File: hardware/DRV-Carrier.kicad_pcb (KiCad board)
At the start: 4 copper layers, 95 x 79.9 mm, 22 parts, among them J1 Conn_01x02, J2 Conn_02x25_Counter_Clockwise

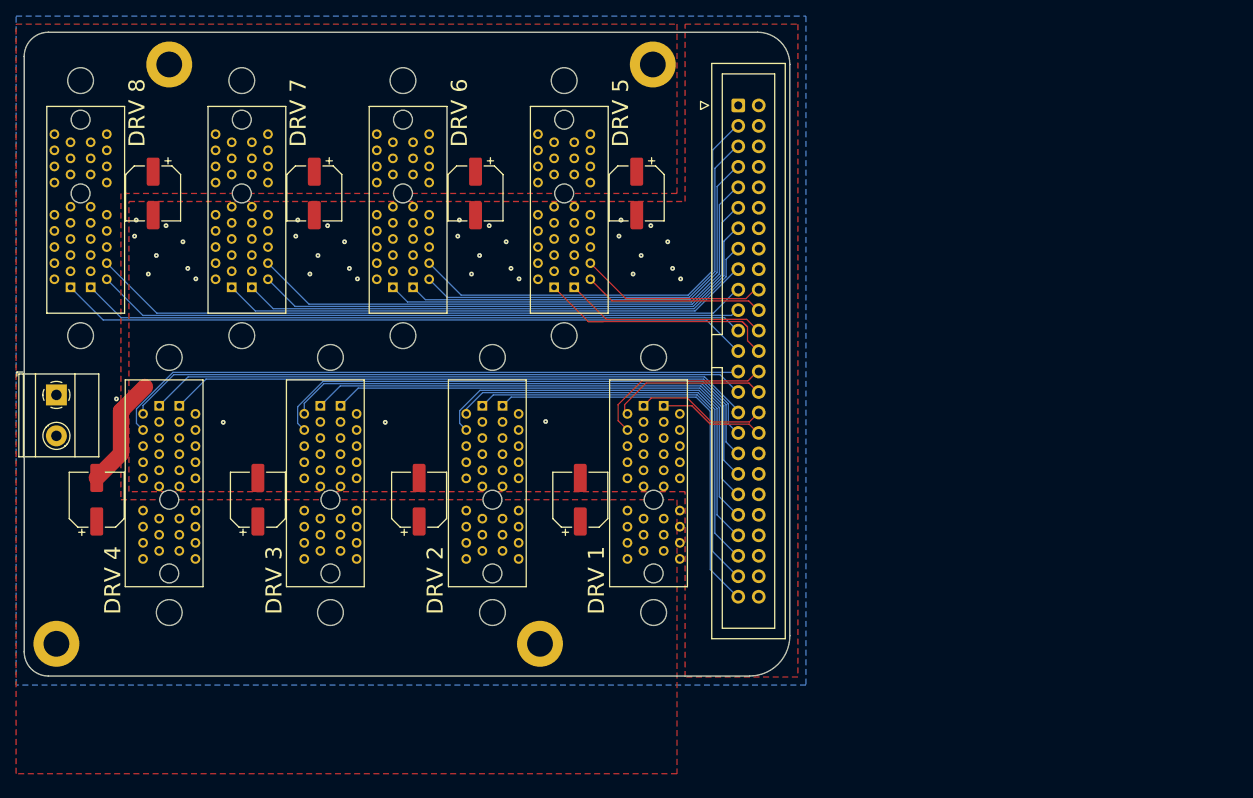
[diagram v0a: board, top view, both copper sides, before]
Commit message: V3 added
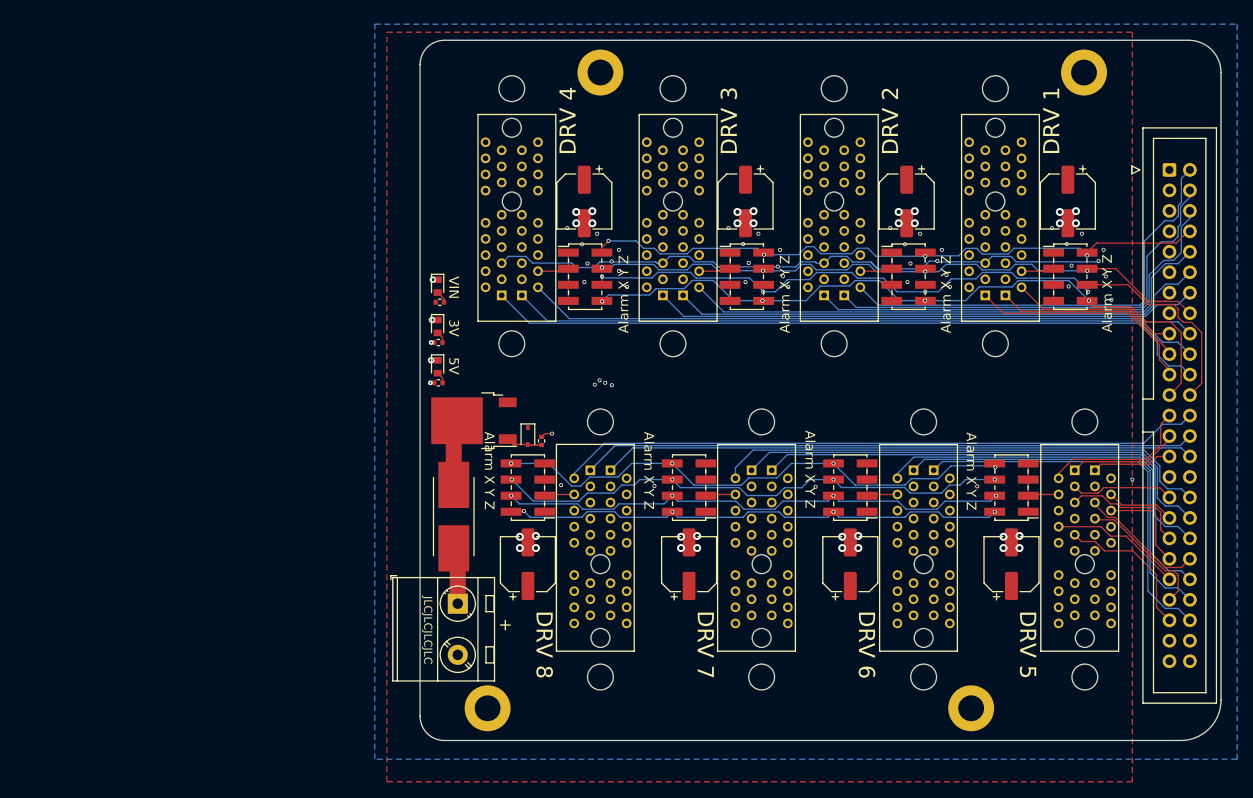
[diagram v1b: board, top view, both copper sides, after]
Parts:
- added D1: 10V, Diode_SMD:D_SOD-323, F.Cu at (107.5, 100.1)
- added D2: LED, PrntrBoardV2:LED_0603_1608Metric, F.Cu at (96.3, 81.5)
- added D3: LED, PrntrBoardV2:LED_0603_1608Metric, F.Cu at (96.3, 86.5)
- added D4: LED, PrntrBoardV2:LED_0603_1608Metric, F.Cu at (96.3, 91.5)
- added F1: Fuse, PrntrBoardV2:2410_FuseFolder, F.Cu at (98.3, 110.1)
- added J_A1: AlarmSelector, Connector_PinHeader_2.00mm:PinHeader_2x04_P2.00mm_Vertical_SMD, F.Cu at (174.8, 80.3)
- added J_A2: AlarmSelector, Connector_PinHeader_2.00mm:PinHeader_2x04_P2.00mm_Vertical_SMD, F.Cu at (154.7, 80.3)
- added J_A3: AlarmSelector, Connector_PinHeader_2.00mm:PinHeader_2x04_P2.00mm_Vertical_SMD, F.Cu at (134.7, 80.3)
- added J_A4: AlarmSelector, Connector_PinHeader_2.00mm:PinHeader_2x04_P2.00mm_Vertical_SMD, F.Cu at (114.6, 80.3)
- added J_A5: AlarmSelector, Connector_PinHeader_2.00mm:PinHeader_2x04_P2.00mm_Vertical_SMD, F.Cu at (167.5, 106.5)
- added J_A6: AlarmSelector, Connector_PinHeader_2.00mm:PinHeader_2x04_P2.00mm_Vertical_SMD, F.Cu at (147.5, 106.5)
- added J_A7: AlarmSelector, Connector_PinHeader_2.00mm:PinHeader_2x04_P2.00mm_Vertical_SMD, F.Cu at (127.5, 106.5)
- added J_A8: AlarmSelector, Connector_PinHeader_2.00mm:PinHeader_2x04_P2.00mm_Vertical_SMD, F.Cu at (107.5, 106.5)
- added LOGO1: Logo_Open_Hardware_Small, Symbol:OSHW-Logo_5.7x6mm_SilkScreen, B.Cu at (97.7, 90.5)
- added Q1: NCE40P40K, Package_TO_SOT_SMD:TO-252-2, F.Cu at (100.8, 98.2)
- added R1: 100k, Resistor_SMD:R_0402_1005Metric, F.Cu at (109.2, 100.7)
- added R2: 10k, Resistor_SMD:R_0402_1005Metric, F.Cu at (96.6, 83.5)
- added R3: 470, Resistor_SMD:R_0402_1005Metric, F.Cu at (96.4, 88.5)
- added R4: 1k, Resistor_SMD:R_0402_1005Metric, F.Cu at (96.4, 93.5)
- J1: value Conn_01x02 -> KF635; footprint TerminalBlock_Phoenix:TerminalBlock_Phoenix_MKDS-1,5-2-5.08_1x02_P5.08mm_Horizontal -> TerminalBlock_MetzConnect:TerminalBlock_MetzConnect_Type701_RT11L02HGLU_1x02_P6.35mm_Horizontal
- moved J1 56.1 mm to (98.8, 120.9)
- moved C1 54.1 mm to (127.5, 116.0)
- moved C2 54.1 mm to (107.5, 116.0)
- moved C4 54.1 mm to (147.5, 116.0)
- moved C5 54.1 mm to (167.5, 116.0)
- moved H3 54.1 mm to (102.5, 133.9)
- moved H4 54.1 mm to (162.5, 133.9)
- moved J2 54.1 mm to (187.1, 67.1)
- moved J_MOT5 54.1 mm to (176.6, 116.0)
- moved J_MOT6 54.1 mm to (156.6, 116.0)
- moved J_MOT7 54.1 mm to (136.5, 116.0)
- moved J_MOT8 54.1 mm to (116.5, 116.0)
- moved C3 53.5 mm to (114.5, 71.0)
- moved C6 53.5 mm to (174.5, 71.0)
- moved C7 53.5 mm to (154.5, 71.0)
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- renumbered J_MOT5 to J_MOT1, J_MOT6 to J_MOT2, J_MOT7 to J_MOT3, J_MOT8 to J_MOT4, J_MOT1 to J_MOT5, J_MOT4 to J_MOT6, J_MOT2 to J_MOT7, J_MOT3 to J_MOT8
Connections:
- J1 pad 1: V_motors -> /IO/Vin
- J2 pad 1: 3.3V -> 5V
- J2 pad 10: MOT_I2C_SCL -> MOT3_DIR
- J2 pad 11: ~MOT7_ALARM -> (no net)
- J2 pad 12: MOT_UART -> MOT3_STEP
- J2 pad 13: MOT7_DIR -> MOT_SPI_MOSI
- J2 pad 14: ~MOT_RESET -> ~MOT3_CS
- J2 pad 15: MOT7_STEP -> MOT_SPI_MISO
- J2 pad 16: MOT_SPI_SCK -> ~Y_ALARM
- J2 pad 17: ~MOT7_CS -> MOT1_DIR
- J2 pad 18: ~MOT_ENABLE -> MOT4_DIR
- J2 pad 19: ~MOT8_ALARM -> MOT1_STEP
- J2 pad 2: GND -> MOT2_DIR
- J2 pad 20: ~MOT5_ALARM -> MOT4_STEP
- J2 pad 21: MOT8_DIR -> ~MOT1_CS
- J2 pad 22: MOT5_DIR -> ~MOT4_CS
- J2 pad 23: MOT8_STEP -> ~MOT_ALARM
- J2 pad 24: MOT5_STEP -> ~X_ALARM
- J2 pad 25: ~MOT8_CS -> MOT5_DIR
- J2 pad 26: ~MOT5_CS -> MOT8_DIR
- J2 pad 27: ~MOT4_ALARM -> MOT5_STEP
- J2 pad 28: ~MOT1_ALARM -> MOT8_STEP
- J2 pad 29: MOT4_DIR -> ~MOT5_CS
- J2 pad 3: ~MOT6_ALARM -> 3.3V
- J2 pad 30: MOT1_DIR -> ~MOT8_CS
- J2 pad 31: MOT4_STEP -> (no net)
- J2 pad 32: MOT1_STEP -> (no net)
- J2 pad 33: ~MOT4_CS -> ~MOT_ENABLE
- J2 pad 34: ~MOT1_CS -> MOT7_DIR
- J2 pad 35: ~MOT3_ALARM -> MOT_SPI_SCK
- J2 pad 36: MOT_SPI_MISO -> MOT7_STEP
- J2 pad 37: MOT3_DIR -> ~MOT_RESET
- J2 pad 38: MOT_SPI_MOSI -> ~MOT7_CS
- J2 pad 39: MOT3_STEP -> MOT_UART_RX
- J2 pad 4: GND -> MOT2_STEP
- J2 pad 40: (no net) -> MOT_UART_TX
- J2 pad 41: ~MOT3_CS -> MOT_I2C_SCL
- J2 pad 42: (no net) -> MOT6_DIR
- J2 pad 43: ~MOT2_ALARM -> CLOCK
- J2 pad 44: (no net) -> MOT6_STEP
- J2 pad 45: MOT2_DIR -> MOT_I2C_SDA
- J2 pad 46: GND -> ~MOT6_CS
- J2 pad 47: MOT2_STEP -> GND
- J2 pad 48: 3.3V -> (no net)
- J2 pad 49: ~MOT2_CS -> GND
- J2 pad 5: MOT6_DIR -> GND
- J2 pad 50: 5V -> 3.3V
- J2 pad 6: MOT_I2C_SDA -> ~MOT2_CS
- J2 pad 7: MOT6_STEP -> (no net)
- J2 pad 8: CLOCK -> ~Z_ALARM
- J2 pad 9: ~MOT6_CS -> (no net)
- J_MOT1 pad A1: ~MOT5_CS -> ~MOT1_CS
- J_MOT1 pad A5: (no net) -> MOT_UART_TX
- J_MOT1 pad A6: MOT_UART -> MOT_UART_RX
- J_MOT1 pad B1: MOT5_STEP -> MOT1_STEP
- J_MOT1 pad B13: 3.3V -> GND
- J_MOT1 pad B2: MOT5_DIR -> MOT1_DIR
- J_MOT1 pad B4: ~MOT5_ALARM -> ~MOT1_ALARM
- J_MOT2 pad A1: ~MOT6_CS -> ~MOT2_CS
- J_MOT2 pad A5: (no net) -> MOT_UART_TX
- J_MOT2 pad A6: MOT_UART -> MOT_UART_RX
- J_MOT2 pad B1: MOT6_STEP -> MOT2_STEP
- J_MOT2 pad B13: 3.3V -> GND
- J_MOT2 pad B2: MOT6_DIR -> MOT2_DIR
- J_MOT2 pad B4: ~MOT6_ALARM -> ~MOT2_ALARM
- J_MOT3 pad A1: ~MOT7_CS -> ~MOT3_CS
- J_MOT3 pad A5: (no net) -> MOT_UART_TX
- J_MOT3 pad A6: MOT_UART -> MOT_UART_RX
- J_MOT3 pad B1: MOT7_STEP -> MOT3_STEP
- J_MOT3 pad B13: 3.3V -> GND
- J_MOT3 pad B2: MOT7_DIR -> MOT3_DIR
- J_MOT3 pad B4: ~MOT7_ALARM -> ~MOT3_ALARM
- J_MOT4 pad A1: ~MOT8_CS -> ~MOT4_CS
- J_MOT4 pad A5: (no net) -> MOT_UART_TX
- J_MOT4 pad A6: MOT_UART -> MOT_UART_RX
- J_MOT4 pad B1: MOT8_STEP -> MOT4_STEP
- J_MOT4 pad B13: 3.3V -> GND
- J_MOT4 pad B2: MOT8_DIR -> MOT4_DIR
- J_MOT4 pad B4: ~MOT8_ALARM -> ~MOT4_ALARM
- J_MOT5 pad A1: ~MOT1_CS -> ~MOT5_CS
- J_MOT5 pad A5: (no net) -> MOT_UART_TX
- J_MOT5 pad A6: MOT_UART -> MOT_UART_RX
- J_MOT5 pad B1: MOT1_STEP -> MOT5_STEP
- J_MOT5 pad B13: GND -> 3.3V
- J_MOT5 pad B2: MOT1_DIR -> MOT5_DIR
- J_MOT5 pad B4: ~MOT1_ALARM -> ~MOT5_ALARM
- J_MOT6 pad A1: ~MOT2_CS -> ~MOT6_CS
- J_MOT6 pad A5: (no net) -> MOT_UART_TX
- J_MOT6 pad A6: MOT_UART -> MOT_UART_RX
- J_MOT6 pad B1: MOT2_STEP -> MOT6_STEP
- J_MOT6 pad B13: GND -> 3.3V
- J_MOT6 pad B2: MOT2_DIR -> MOT6_DIR
- J_MOT6 pad B4: ~MOT2_ALARM -> ~MOT6_ALARM
- J_MOT7 pad A1: ~MOT3_CS -> ~MOT7_CS
- J_MOT7 pad A5: (no net) -> MOT_UART_TX
- J_MOT7 pad A6: MOT_UART -> MOT_UART_RX
- J_MOT7 pad B1: MOT3_STEP -> MOT7_STEP
- J_MOT7 pad B13: GND -> 3.3V
- J_MOT7 pad B2: MOT3_DIR -> MOT7_DIR
- J_MOT7 pad B4: ~MOT3_ALARM -> ~MOT7_ALARM
- J_MOT8 pad A1: ~MOT4_CS -> ~MOT8_CS
- J_MOT8 pad A5: (no net) -> MOT_UART_TX
- J_MOT8 pad A6: MOT_UART -> MOT_UART_RX
- J_MOT8 pad B1: MOT4_STEP -> MOT8_STEP
- J_MOT8 pad B13: GND -> 3.3V
- J_MOT8 pad B2: MOT4_DIR -> MOT8_DIR
- J_MOT8 pad B4: ~MOT4_ALARM -> ~MOT8_ALARM
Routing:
- net MOT_UART_RX: track 0.00 -> 222.3 mm, vias 0 -> 4
- net MOT_UART_TX: track 0.00 -> 217.9 mm, vias 0 -> 4
- net MOT_UART: track 196.2 -> 0.00 mm, vias 4 -> 0
- net ~X_ALARM: track 0.00 -> 190.3 mm, vias 0 -> 9
- net ~Z_ALARM: track 0.00 -> 181.9 mm, vias 0 -> 9
- net ~MOT_ALARM: track 0.00 -> 181.1 mm, vias 0 -> 9
- net ~Y_ALARM: track 0.00 -> 180.0 mm, vias 0 -> 9
- net ~MOT8_ALARM: track 82.0 -> 9.52 mm
- net ~MOT4_ALARM: track 79.4 -> 9.45 mm
- net ~MOT7_ALARM: track 69.1 -> 9.51 mm
- net ~MOT3_ALARM: track 65.5 -> 9.52 mm
- net ~MOT6_ALARM: track 57.3 -> 9.61 mm
- net MOT_SPI_MOSI: track 162.9 -> 209.0 mm, vias 4 -> 5
- net ~MOT2_ALARM: track 53.4 -> 9.59 mm
- net ~MOT_RESET: track 184.3 -> 218.1 mm
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- removed copper zone on F.Cu, net GND
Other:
- board size 95 x 79.9 mm -> 99.4 x 86.9 mm
- board text added: "+"
- board text added: "1"
- board text added: "2"
- board text added: "3"
- board text added: "3V"
- board text added: "4"
- board text added: "5"
- board text added: "5V"
- board text added: "6"
- board text added: "7"
- board text added: "8"
- board text added: "Alarm X Y Z"
- board text added: "JLCJLCJLCJLC"
- board text added: "Taco Lion Motor Driver Board"
- board text added: "VIN"
- board text removed: "Driver Card Carrier Board"
